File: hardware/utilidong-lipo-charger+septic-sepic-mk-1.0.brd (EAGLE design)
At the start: 32 x 30 mm, 31 parts, among them IC1 LT1610, IC2 MCP73831, Q1 N-MOSFET

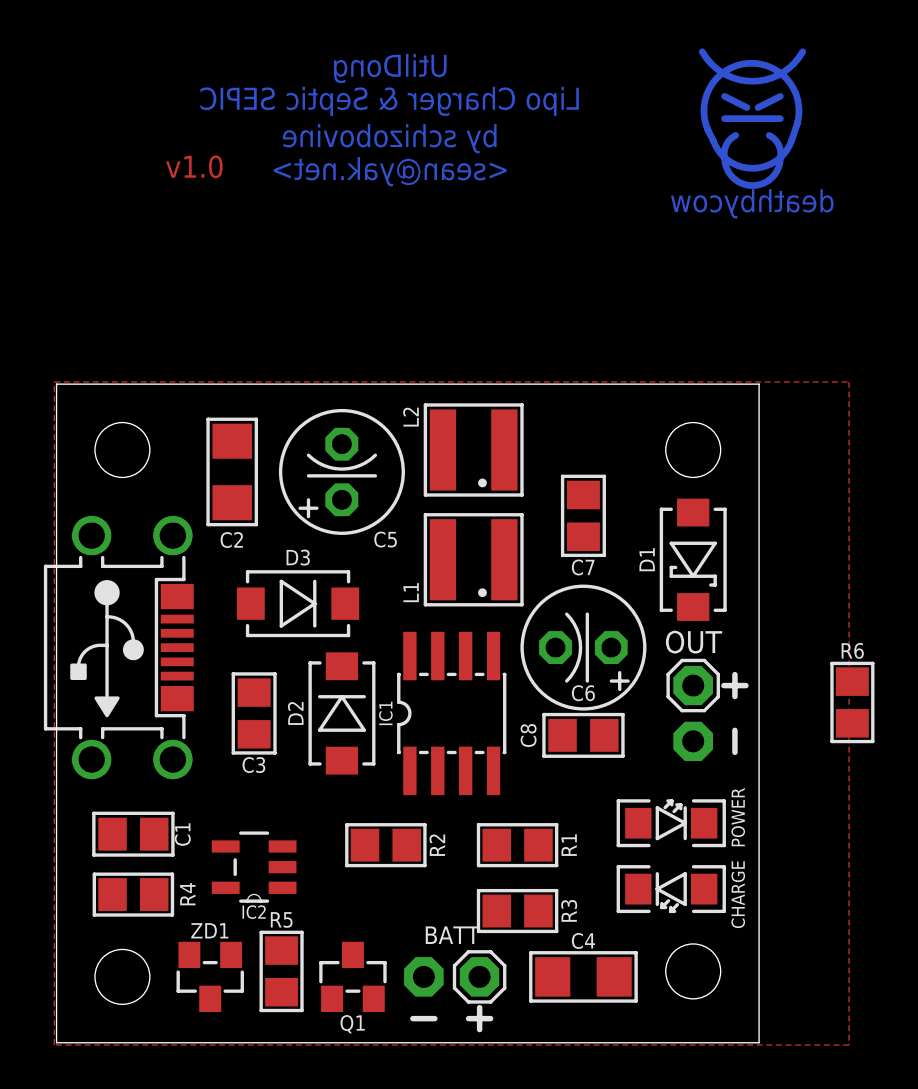
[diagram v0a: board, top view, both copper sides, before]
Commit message: twiddling around
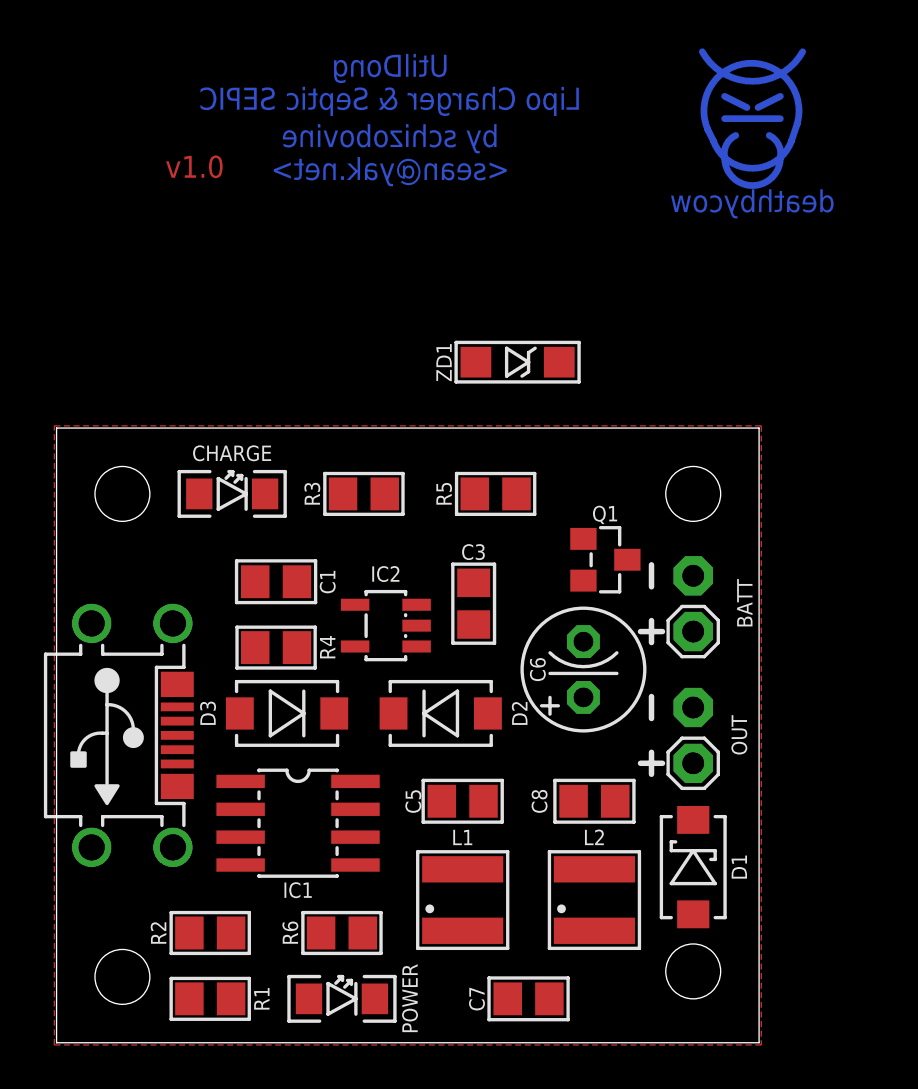
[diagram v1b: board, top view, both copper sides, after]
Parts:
- removed C2, C4: 10uF, A_butts:C1206
- C1, C3: value 100nF -> 4.7uF
- C5: value 22uF -> 10uF; device A_butts:E2,5-6 -> A_butts:C0805
- ZD1: device A_butts:SOT23 -> A_butts:SOD123-ZENER
- moved ZD1 31.3 mm to (21.0, 31.0), turned to 0 degrees
- moved CHARGE 26.9 mm to (8.00, 25.0), turned to 0 degrees
- moved R6 25.5 mm to (13.0, 5.00), turned to 0 degrees
- moved R5 23.8 mm to (20.0, 25.0), turned to 0 degrees
- moved Q1 22.2 mm to (25.0, 22.0), turned to 270 degrees
- moved C7 22.1 mm to (21.5, 2.00), turned to 180 degrees
- moved L2 21.2 mm to (24.5, 6.50), turned to 90 degrees
- moved BATT 20.2 mm to (29.0, 20.0), turned to 270 degrees
- moved R3 20.2 mm to (14.0, 25.0), turned to 0 degrees
- moved POWER 17.0 mm to (13.0, 2.00)
- moved C5 16.0 mm to (18.5, 11.0), turned to 0 degrees
- moved R1 15.7 mm to (7.00, 2.00)
- moved L1 15.5 mm to (18.5, 6.50), turned to 90 degrees
- moved D1 14.0 mm to (29.0, 8.00), turned to 90 degrees
- moved C1 13.2 mm to (10.0, 21.0)
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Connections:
- net 5V: no longer C2.1
- net GND: now also C5.2, ZD1.A; no longer C2.2, C4.2, C5.-, ZD1.1, ZD1.2
- net N$11: now also ZD1.C; no longer ZD1.3
- net VBATT+: no longer C4.1
- net VIN: now also C5.1; no longer C5.+
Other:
- board size 32 x 30 mm -> 32 x 28 mm
